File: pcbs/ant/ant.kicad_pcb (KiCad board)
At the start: 2 copper layers, 101.3 x 95.6 mm, 16 parts, among them SW1 SW_PUSH, SW10 SW_PUSH, SW11 SW_PUSH, SW12 SW_PUSH, SW13 SW_PUSH, SW2 SW_PUSH, SW3 SW_PUSH, SW4 SW_PUSH, SW5 SW_PUSH, SW6 SW_PUSH, SW7 SW_PUSH, SW8 SW_PUSH, SW9 SW_PUSH, U1 ProMicro

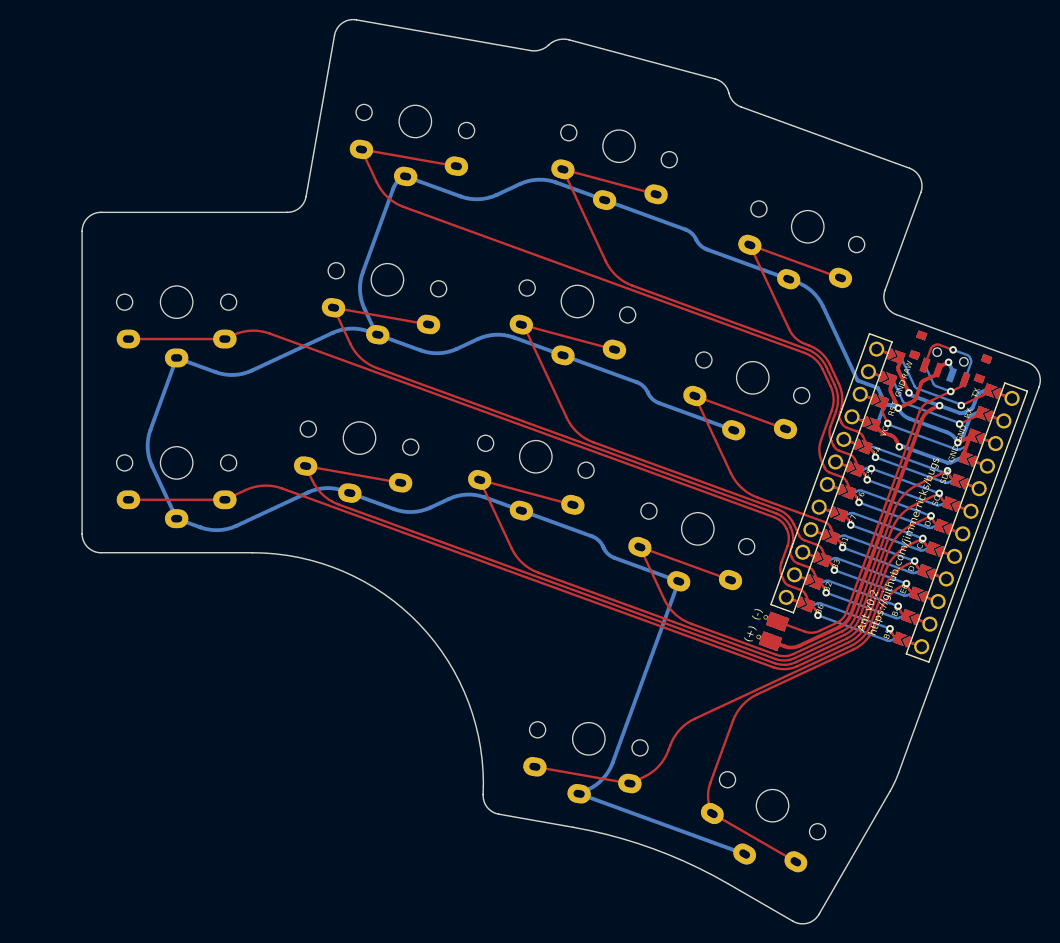
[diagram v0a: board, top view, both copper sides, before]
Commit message: Minor edits
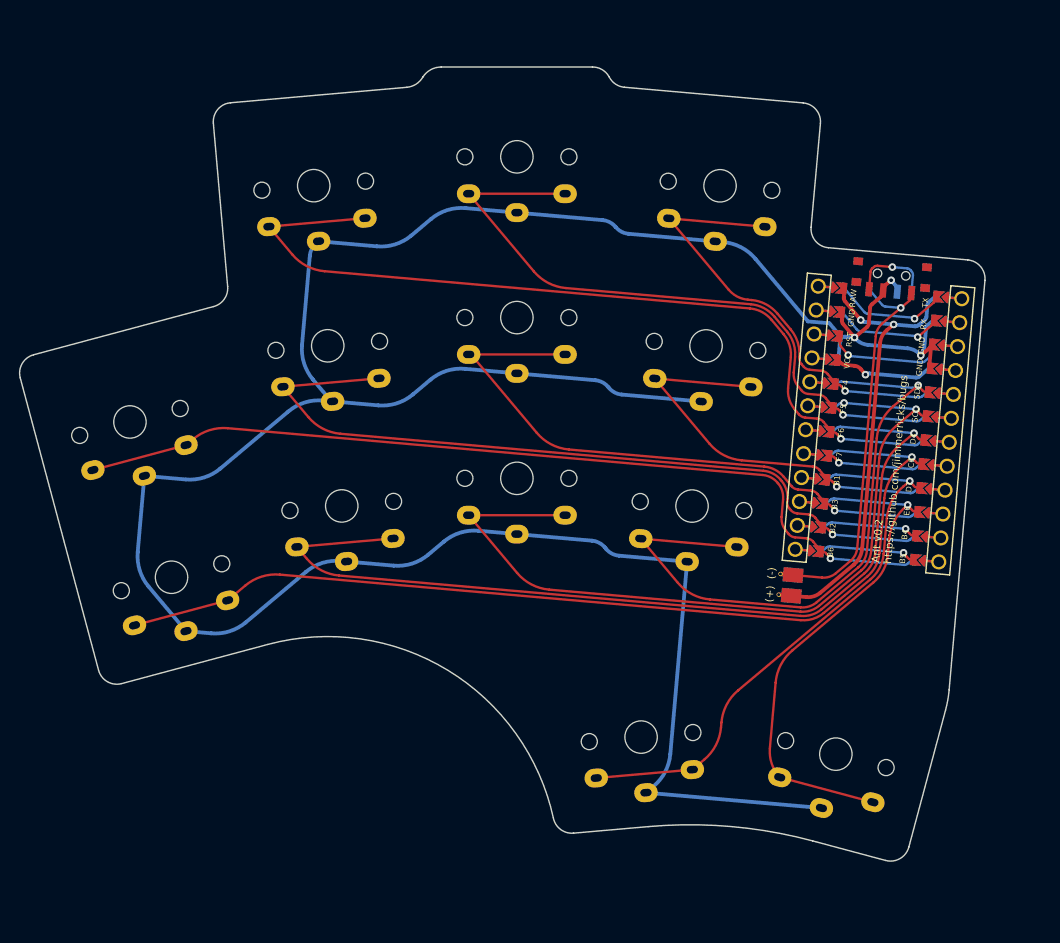
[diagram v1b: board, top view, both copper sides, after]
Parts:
- moved SW4 13.6 mm to (39.0, 103.1), turned to 15 degrees
- moved SW1 12.7 mm to (58.5, 78.1), turned to 5 degrees
- moved SW8 12.1 mm to (43.4, 119.5), turned to 15 degrees
- moved SW2 10.9 mm to (80.0, 75.1), turned to 0 degrees
- moved PSW1 10.7 mm to (119.6, 87.5), turned to 175 degrees
- moved SW3 10.2 mm to (101.5, 78.1), turned to -5 degrees
- moved SW5 9.41 mm to (60.0, 95.0), turned to 5 degrees
- moved SW13 8.64 mm to (113.7, 138.2), turned to -15 degrees
- moved U1 8.11 mm to (118.2, 103.3), turned to -5 degrees
- moved SW9 7.42 mm to (61.5, 112.0), turned to 5 degrees
- moved SW6 6.63 mm to (80.0, 92.1), turned to 0 degrees
- moved SW7 5.99 mm to (100.0, 95.1), turned to -5 degrees
- moved SW12 5.53 mm to (93.1, 136.4), turned to 5 degrees
- moved BT1 5.23 mm to (109.1, 120.4), turned to 85 degrees
- moved SW10 3.04 mm to (80.0, 109.1), turned to 0 degrees
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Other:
- board size 101.3 x 95.6 mm -> 102.1 x 84 mm
